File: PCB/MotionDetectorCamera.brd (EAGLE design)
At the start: 41.9 x 32.6 mm, 185 parts, among them J1 JUMPER-SOLDER, J10 MICROSD-SOCKET, J11 USB-C-JACK, J2 JUMPER-SOLDER, J3 JUMPER-SOLDER, J4 JUMPER-SOLDER, J5 JST-SM02B-SRSS-TB, J6 JUMPER-SOLDER, J7 JUMPER-SOLDER, J8 JUMPER-SOLDER, J9 S-MOUNT-LENS-HOLDERM12LENSES-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, Q1 PMOS-NEXPERIA-SOT1220, Q2 PMOS-NEXPERIA-SOT1220, Q3 PMOS-NEXPERIA-SOT1220, U1 TI-TPS2116, U10 TI-TPS22919DCK, U11 TI-TPS62A01, U13 TI-TPS22919DCK, U14 TI-TPS22919DCK, U15 TI-MSP430FR2422IRHL, U16 NXP-NTB0102, U17 NXP-NTB0102, U18 PANASONIC-EKMB110711X, U19 LATTICE-ICE40HX4K-BG121, U2 DIODESINC-AP7350, U20 WINBOND-W25Q40EW, U21 NEXPERIA-74LVC1G98-OR-INV-INP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, U22 NEXPERIA-74LVC1G98-BUFFER, U23 ON-AR0330CS1C12SPKA0, U24 ALLIANCE-AS4C8M16MSA-6BIN, U25 STM-STM32F730, U26 DIODESINC-DT1446-04V-7, U27 NEXPERIA-74LVC1G98-BUFFER, U3 NEXPERIA-74LVC1G98-NOR, U4 MICROCHIP-MCP7383X, U5 EATON-STN101, U6 TI-TPS62A01, U7 TI-TPS62A01, U9 TI-TPS22919DCK, X1 EPSON-FC-135, X2 SITIME-SIT8021, X3 SITIME-SIT8021

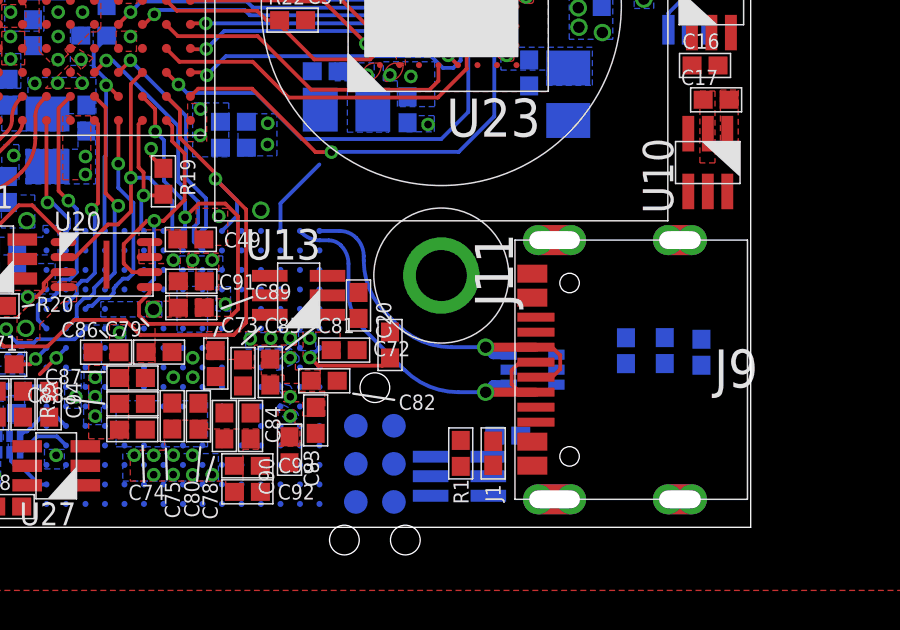
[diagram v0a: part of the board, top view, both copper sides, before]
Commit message: Layout progress
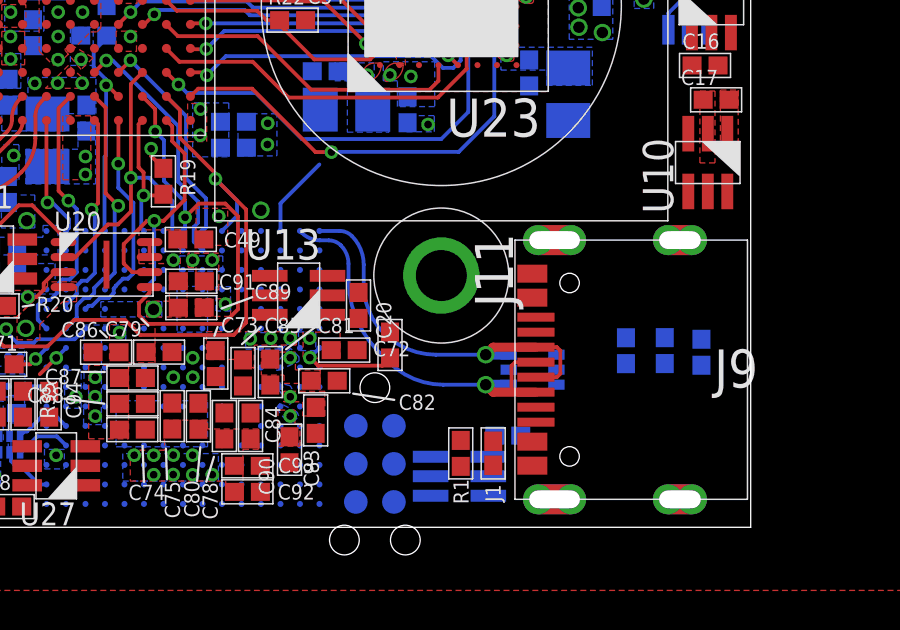
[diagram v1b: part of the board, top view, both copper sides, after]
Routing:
- net USB_D+: track 12.5 -> 13.1 mm

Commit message: Layout progress
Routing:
- net VDD_B: track 11.3 -> 0.00 mm
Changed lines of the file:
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@@
 <grid distance="10" unitdist="mil" unit="mil" style="lines" multiple="1" display="no" altdistance="0.00254" altunitdist="mm" altunit="mil"/>
 <layers>
-<layer number="1" name="Top" color="4" fill="1" visible="yes" active="yes"/>
+<layer number="1" name="Top" color="4" fill="1" visible="no" active="yes"/>
 <layer number="2" name="Ground" color="16" fill="1" visible="no" active="yes"/>
 <layer number="3" name="Route3" color="17" fill="1" visible="no" active="no"/>
@@
 <layer number="13" name="Route13" color="21" fill="1" visible="no" active="no"/>
 <layer number="14" name="Route14" color="22" fill="1" visible="no" active="no"/>
-<layer number="15" name="Power" color="42" fill="1" visible="no" active="yes"/>
+<layer number="15" name="Power" color="42" fill="1" visible="yes" active="yes"/>
 <layer number="16" name="Bottom" color="1" fill="1" visible="no" active="yes"/>
-<layer number="17" name="Pads" color="2" fill="1" visible="yes" active="yes"/>
+<layer number="17" name="Pads" color="2" fill="1" visible="no" active="yes"/>
 <layer number="18" name="Vias" color="2" fill="1" visible="yes" active="yes"/>
 <layer number="19" name="Unrouted" color="6" fill="1" visible="no" active="yes"/>
-<layer number="20" name="Dimension" color="24" fill="1" visible="yes" active="yes"/>
-<layer number="21" name="tPlace" color="7" fill="1" visible="yes" active="yes"/>
+<layer number="20" name="Dimension" color="24" fill="1" visible="no" active="yes"/>
+<layer number="21" name="tPlace" color="7" fill="1" visible="no" active="yes"/>
 <layer number="22" name="bPlace" color="7" fill="1" visible="no" active="yes"/>
-<layer number="23" name="tOrigins" color="15" fill="1" visible="yes" active="yes"/>
+<layer number="23" name="tOrigins" color="15" fill="1" visible="no" active="yes"/>
 <layer number="24" name="bOrigins" color="15" fill="1" visible="no" active="yes"/>
-<layer number="25" name="tNames" color="7" fill="1" visible="yes" active="yes"/>
+<layer number="25" name="tNames" color="7" fill="1" visible="no" active="yes"/>
 <layer number="26" name="bNames" color="7" fill="1" visible="no" active="yes"/>
-<layer number="27" name="tValues" color="7" fill="1" visible="yes" active="yes"/>
+<layer number="27" name="tValues" color="7" fill="1" visible="no" active="yes"/>
 <layer number="28" name="bValues" color="7" fill="1" visible="no" active="yes"/>
-<layer number="29" name="tStop" color="7" fill="3" visible="yes" active="yes"/>
+<layer number="29" name="tStop" color="7" fill="3" visible="no" active="yes"/>
 <layer number="30" name="bStop" color="7" fill="6" visible="no" active="yes"/>
-<layer number="31" name="tCream" color="7" fill="4" visible="yes" active="yes"/>
+<layer number="31" name="tCream" color="7" fill="4" visible="no" active="yes"/>
 <layer number="32" name="bCream" color="7" fill="5" visible="no" active="yes"/>
-<layer number="33" name="tFinish" color="6" fill="3" visible="yes" active="yes"/>
+<layer number="33" name="tFinish" color="6" fill="3" visible="no" active="yes"/>
 <layer number="34" name="bFinish" color="6" fill="6" visible="no" active="yes"/>
-<layer number="35" name="tGlue" color="7" fill="4" visible="yes" active="yes"/>
+<layer number="35" name="tGlue" color="7" fill="4" visible="no" active="yes"/>
 <layer number="36" name="bGlue" color="7" fill="5" visible="no" active="yes"/>
-<layer number="37" name="tTest" color="7" fill="1" visible="yes" active="yes"/>
+<layer number="37" name="tTest" color="7" fill="1" visible="no" active="yes"/>
 <layer number="38" name="bTest" color="7" fill="1" visible="no" active="yes"/>
 <layer number="39" name="tKeepout" color="4" fill="11" visible="no" active="yes"/>
 <layer number="40" name="bKeepout" color="1" fill="11" visible="no" active="yes"/>
-<layer number="41" name="tRestrict" color="4" fill="10" visible="yes" active="yes"/>
+<layer number="41" name="tRestrict" color="4" fill="10" visible="no" active="yes"/>
 <layer number="42" name="bRestrict" color="1" fill="10" visible="no" active="yes"/>
 <layer number="43" name="vRestrict" color="2" fill="10" visible="no" active="yes"/>
@@
 <via x="36.910221875" y="16.49221875" extent="1-16" drill="0.381" grouprefs="_VDD_B_CONTROL"/>
 <via x="36.1279" y="16.67001875" extent="1-16" drill="0.381" grouprefs="_VDD_B_CONTROL"/>
-<wire x1="36.910221875" y1="16.49221875" x2="40.7589125" y2="17.70930625" width="0.635" layer="15"/>
-<wire x1="40.7589125" y1="17.70930625" x2="36.1279" y2="16.67001875" width="0.635" layer="15"/>
-<wire x1="36.10758125" y1="17.317721875" x2="36.74628125" y2="17.2212875" width="0.635" layer="15"/>
-<wire x1="36.74628125" y1="17.2212875" x2="36.1279" y2="16.67001875" width="0.635" layer="15"/>
-<wire x1="36.10758125" y1="17.317721875" x2="37.097209375" y2="17.209559375" width="0.635" layer="15"/>
 <contactref element="C8" pad="1"/>
 <contactref element="C11" pad="1"/>
@@
 <wire x1="25.916" y1="29.437740625" x2="24.865703125" y2="30.355546875" width="0" layer="19" extent="16-16"/>
 <wire x1="26.385140625" y1="28.652059375" x2="25.916" y2="29.437740625" width="0" layer="19" extent="1-16"/>
+<wire x1="26.385140625" y1="27.172059375" x2="26.385140625" y2="28.652059375" width="0" layer="19" extent="1-1"/>
+<wire x1="27.590375" y1="27.4656" x2="26.385140625" y2="27.172059375" width="0" layer="19" extent="1-1"/>
 <wire x1="25.192578125" y1="25.960959375" x2="26.385140625" y2="27.172059375" width="0" layer="19" extent="1-16"/>
 <wire x1="23.712578125" y1="25.960959375" x2="25.192578125" y2="25.960959375" width="0" layer="19" extent="16-16"/>
 <wire x1="23.266496875" y1="27.012225" x2="23.712578125" y2="25.960959375" width="0" layer="19" extent="16-16"/>
 <wire x1="36.10758125" y1="17.317721875" x2="27.590375" y2="27.4656" width="0" layer="19" extent="1-1"/>
+<wire x1="36.1279" y1="16.67001875" x2="36.10758125" y2="17.317721875" width="0" layer="19" extent="1-1"/>
+<wire x1="36.889378125" y1="17.368759375" x2="36.10758125" y2="17.317721875" width="0" layer="19" extent="16-16"/>
+<wire x1="36.910221875" y1="16.49221875" x2="36.1279" y2="16.67001875" width="0" layer="19" extent="1-1"/>
 </signal>
 <signal name="VDD_B_1V8">
@@
 <wire x1="33.2105" y1="21.5555" x2="32.1945" y2="21.5555" width="0.635" layer="15"/>
 <wire x1="32.1945" y1="21.5555" x2="31.115" y2="20.476" width="0.635" layer="15"/>
-<wire x1="31.62808125" y1="17.63104375" x2="31.62808125" y2="17.295759375" width="0.508" layer="15"/>
 <contactref element="J10" pad="VDD"/>
 <contactref element="C68" pad="1"/>
@@
 <vertex x="32.766" y="23.434040625"/>
 </polygon>
-<wire x1="40.424659375" y1="11.19671875" x2="41.074659375" y2="11.19671875" width="0" layer="19" extent="1-1"/>
-<wire x1="34.0472" y1="18.657" x2="40.424659375" y2="11.19671875" width="0" layer="19" extent="1-1"/>
+<wire x1="34.397946875" y1="18.985021875" x2="34.0472" y2="18.657" width="0" layer="19" extent="1-1"/>
+<wire x1="34.0472" y1="19.957" x2="34.397946875" y2="19.625103125" width="0" layer="19" extent="1-1"/>
 <wire x1="32.7472" y1="19.957" x2="34.0472" y2="19.957" width="0" layer="19" extent="1-1"/>
+<wire x1="32.538828125" y1="20.750321875" x2="32.7472" y2="19.957" width="0" layer="19" extent="1-1"/>
+<wire x1="32.477284375" y1="21.42088125" x2="32.538828125" y2="20.750321875" width="0" layer="19" extent="16-16"/>
+<wire x1="32.20645" y1="22.718821875" x2="32.477284375" y2="21.42088125" width="0" layer="19" extent="16-16"/>
 <wire x1="31.115" y1="20.476" x2="32.538828125" y2="20.750321875" width="0" layer="19" extent="1-15"/>
 <wire x1="29.4972" y1="18.657" x2="31.115" y2="20.476" width="0" layer="19" extent="1-15"/>
-<wire x1="31.62808125" y1="17.63104375" x2="29.4972" y2="18.007" width="0" layer="19" extent="1-15"/>
+<wire x1="28.95091875" y1="18.45818125" x2="29.4972" y2="18.657" width="0" layer="19" extent="1-1"/>
+<wire x1="29.4972" y1="18.007" x2="29.4972" y2="18.657" width="0" layer="19" extent="1-1"/>
+<wire x1="27.93005" y1="18.527825" x2="28.95091875" y2="18.45818125" width="0" layer="19" extent="1-1"/>
+<wire x1="27.98481875" y1="18.847859375" x2="27.93005" y2="18.527825" width="0" layer="19" extent="1-16"/>
 <wire x1="29.4972" y1="15.407" x2="29.4972" y2="18.007" width="0" layer="19" extent="1-1"/>
+<wire x1="29.070459375" y1="15.073421875" x2="29.4972" y2="15.407" width="0" layer="19" extent="1-1"/>
+<wire x1="28.105" y1="15.20295625" x2="29.070459375" y2="15.073421875" width="0" layer="19" extent="16-16"/>
+<wire x1="29.257521875" y1="13.920259375" x2="29.070459375" y2="15.073421875" width="0" layer="19" extent="16-16"/>
+<wire x1="40.424659375" y1="11.19671875" x2="34.0472" y2="18.657" width="0" layer="19" extent="1-1"/>
+<wire x1="41.074659375" y1="11.19671875" x2="40.424659375" y2="11.19671875" width="0" layer="19" extent="1-1"/>
 <wire x1="6.80935" y1="9.057684375" x2="28.105" y2="15.20295625" width="0" layer="19" extent="16-16"/>
+<wire x1="5.746746875" y1="8.2338" x2="6.090928125" y2="9.057684375" width="0" layer="19" extent="1-1"/>
+<wire x1="6.48033125" y1="8.09901875" x2="5.746746875" y2="8.2338" width="0" layer="19" extent="1-16"/>
+<wire x1="6.193234375" y1="6.911915625" x2="6.48033125" y2="8.09901875" width="0" layer="19" extent="1-16"/>
 </signal>
 <signal name="VDD_B_2V8_IMG_SD_EN">
